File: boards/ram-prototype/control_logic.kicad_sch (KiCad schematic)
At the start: 18 parts, among them U1 74LVC1G04, U2 74LVC1G04, U3 74LVC1G04, U4 74LVC1G08, U5 74LVC1G08, U6 74LVC1G08

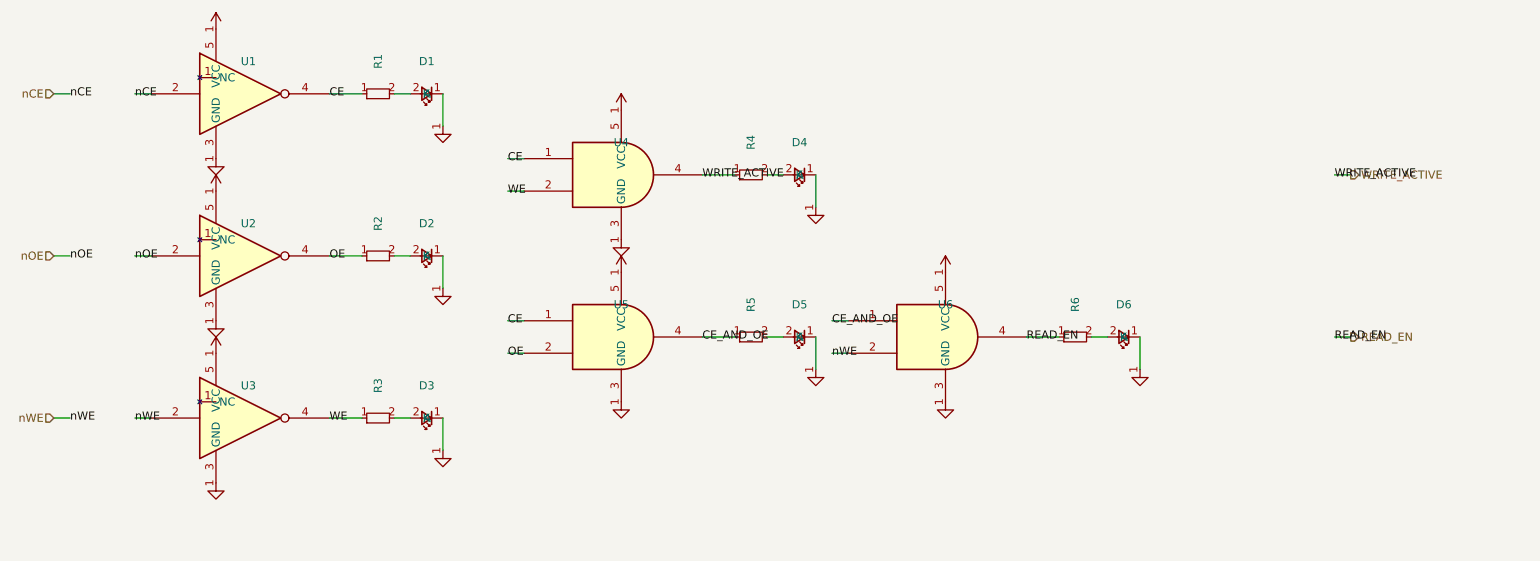
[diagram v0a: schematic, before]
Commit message: Schematic is starting to look good
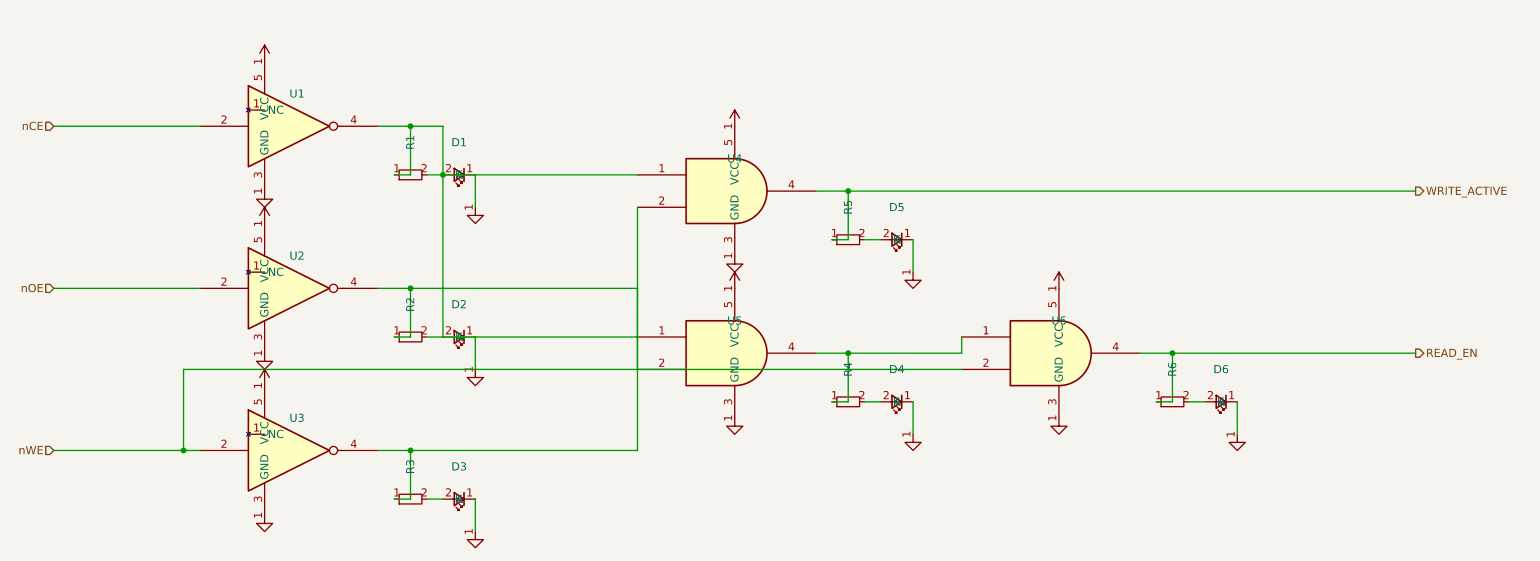
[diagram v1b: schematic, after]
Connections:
- net CE is gone; now on an unnamed net: R1.1, U1.4, U4.1, U5.1
- net WE is gone; now on an unnamed net: R3.1, U3.4, U4.2
- net WRITE_ACTIVE: now also R5.1; no longer R4.1
- net at D1.2 (A), R1.2: now also D2.2 (A), R2.2
- net CE_AND_OE: no longer names the net of U5.4, U6.1
- net CE_AND_OE: now also R4.1; no longer R5.1
- net OE: no longer names the net of R2.1, U2.4, U5.2
